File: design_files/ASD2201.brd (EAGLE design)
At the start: 22.5 x 21.3 mm, 13 parts, among them J1 DF12-32-DP, J2 DF12-32-DS, J3 DM3D-SF, U1 XC6217A33, U2 TXB0104

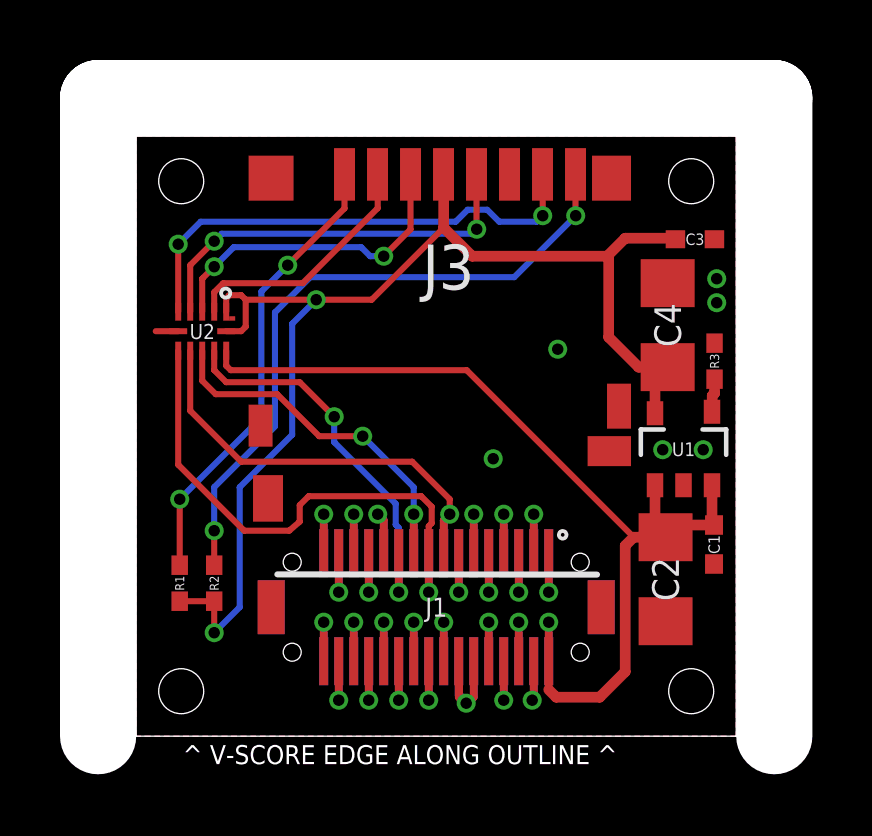
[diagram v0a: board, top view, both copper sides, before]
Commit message: update format
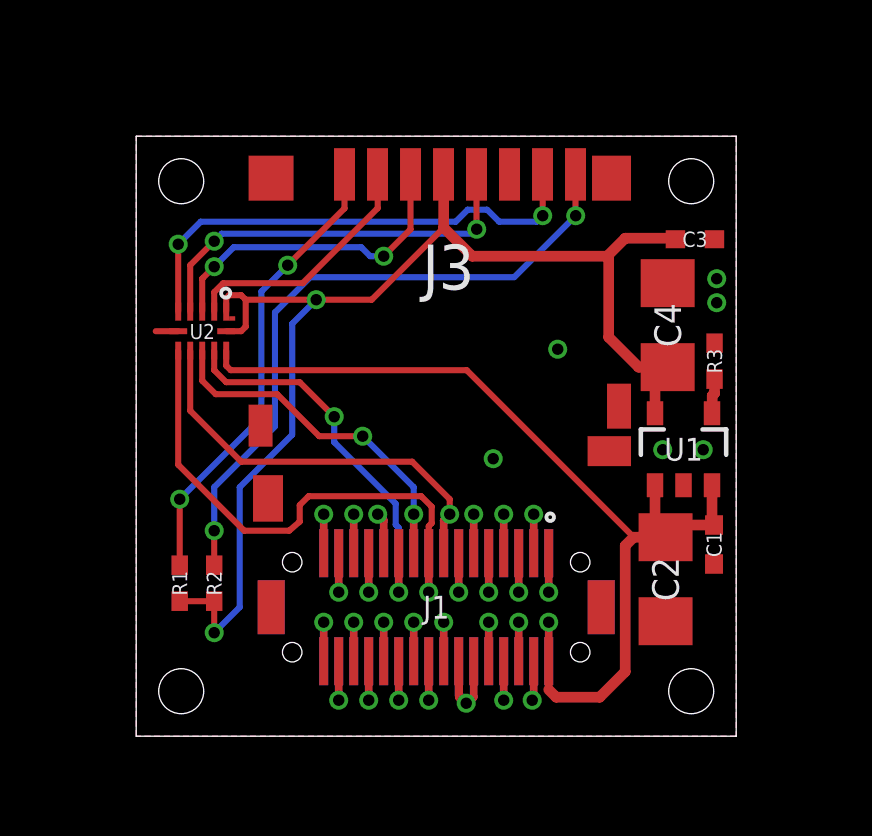
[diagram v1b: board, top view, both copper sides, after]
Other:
- board size 22.5 x 21.3 mm -> 20 x 20 mm
- board text added: "TinyCircuits.com"
- board text removed: "Tiny-Circuits.com"
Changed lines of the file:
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@@
 <setting verticaltext="up"/>
 </settings>
-<grid distance="0.5" unitdist="mm" unit="mm" style="lines" multiple="1" display="yes" altdistance="0.025" altunitdist="inch" altunit="inch"/>
+<grid distance="0.1" unitdist="mm" unit="mm" style="lines" multiple="1" display="yes" altdistance="0.025" altunitdist="inch" altunit="inch"/>
 <layers>
 <layer number="1" name="Top" color="4" fill="1" visible="yes" active="yes"/>
@@
 <hole x="11.5" y="11.5" drill="1.5"/>
 <dimension x1="10" y1="30" x2="10" y2="10" x3="5.95" y3="20" layer="48"/>
-<wire x1="31.27" y1="31.27" x2="31.27" y2="10" width="2.54" layer="46"/>
-<wire x1="8.73" y1="10" x2="8.73" y2="31.27" width="2.54" layer="46"/>
-<wire x1="8.73" y1="31.27" x2="31.27" y2="31.27" width="2.54" layer="46"/>
+<wire x1="31.27" y1="31.27" x2="31.27" y2="10" width="2.54" layer="41"/>
+<wire x1="8.73" y1="10" x2="8.73" y2="31.27" width="2.54" layer="41"/>
+<wire x1="8.73" y1="31.27" x2="31.27" y2="31.27" width="2.54" layer="41"/>
 <text x="40.3098" y="14.837396875" size="0.4572" layer="48" ratio="10">Released under the Creative Commons Attribution Share-Alike 3.0 License</text>
 <text x="40.3098" y="14.075396875" size="0.4572" layer="48" ratio="10">http://creativecommons.org/licenses/by-sa/3.0</text>
@@
 <rectangle x1="17.853659375" y1="28.0924" x2="18.072096875" y2="28.097475" layer="22"/>
 <rectangle x1="17.879059375" y1="28.097478125" x2="18.041615625" y2="28.102559375" layer="22"/>
-<text x="20" y="23.6" size="0.762" layer="22" rot="MR180" align="bottom-center">Tiny-Circuits.com</text>
+<text x="20" y="23.6" size="0.762" layer="22" rot="MR180" align="bottom-center">TinyCircuits.com</text>
 <text x="20" y="22.1" size="0.762" layer="22" rot="MR180" align="bottom-center">ASD2201 - Rev2</text>
 <text x="20" y="20.6" size="0.762" layer="22" rot="MR180" align="bottom-center">microSD TinyShield</text>
-<text x="11.55" y="9.0678" size="0.635" layer="20">^ V-SCORE EDGE ALONG OUTLINE ^</text>
+<text x="11.55" y="9.0678" size="0.635" layer="41">^ V-SCORE EDGE ALONG OUTLINE ^</text>
 </plain>
 <attributes>
@@
 <param name="psElongationOffset" value="100"/>
 <param name="mvStopFrame" value="1"/>
-<param name="mvCreamFrame" value="0.1"/>
+<param name="mvCreamFrame" value="0.05"/>
 <param name="mlMinStopFrame" value="4mil"/>
 <param name="mlMaxStopFrame" value="4mil"/>
-<param name="mlMinCreamFrame" value="1mil"/>
+<param name="mlMinCreamFrame" value="0mil"/>
 <param name="mlMaxCreamFrame" value="4mil"/>
 <param name="mlViaStopLimit" value="25mil"/>
@@
 <attribute name="PARTNO" value="AS-ITM-00048" x="12.2" y="23.5" size="1.778" layer="27" rot="R180" display="off"/>
 <attribute name="VALUE" value="TXB0104" x="12.2" y="23.5" size="1.778" layer="27" rot="R180" display="off"/>
+<attribute name="PNPROTATION" value="0" x="12.2" y="23.5" size="1.778" layer="27" rot="R180" display="off"/>
 </element>
 <element name="J3" library="tinycircuits" package="SD_CARD" value="DM3D-SF" x="20.2438" y="28.7274" rot="R180">
 <attribute name="PARTNO" value="AS-ITM-00047" x="20.2438" y="28.7274" size="1.778" layer="27" rot="R180" display="off"/>
 <attribute name="VALUE" value="DM3D-SF" x="20.2438" y="28.7274" size="1.778" layer="27" rot="R180" display="off"/>
+<attribute name="PNPROTATION" value="270" x="20.2438" y="28.7274" size="1.778" layer="27" rot="R180" display="off"/>
 </element>
 <element name="U1" library="tinycircuits" package="SOT-25" value="XC6217A33" x="28.243859375" y="19.564665625">
 <attribute name="PARTNO" value="AS-ITM-00249" x="28.243859375" y="19.564665625" size="1.778" layer="27" display="off"/>
 <attribute name="VALUE" value="XC6217A33" x="28.243859375" y="19.564665625" size="1.778" layer="27" display="off"/>
+<attribute name="PNPROTATION" value="270" x="28.243859375" y="19.564665625" size="1.778" layer="27" display="off"/>
 </element>
 <element name="C3" library="tinycircuits" package="C0402" value="0.1uF" x="28.624478125" y="26.56481875">
@@
 <wire x1="29.278" y1="21.428" x2="29.2" y2="21.35" width="0.3556" layer="1"/>
 <wire x1="29.2" y1="21.35" x2="29.2" y2="20.82080625" width="0.3556" layer="1"/>
-<wire x1="29.2" y1="20.82080625" x2="29.193859375" y2="20.814665625" width="0.3556" layer="1"/>
+<wire x1="29.2" y1="20.82080625" x2="29.193859375" y2="20.764665625" width="0.3556" layer="1"/>
 </signal>
 </signals>
